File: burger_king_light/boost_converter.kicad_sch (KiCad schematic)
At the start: 14 parts, among them IC1 TPS55340PWPR

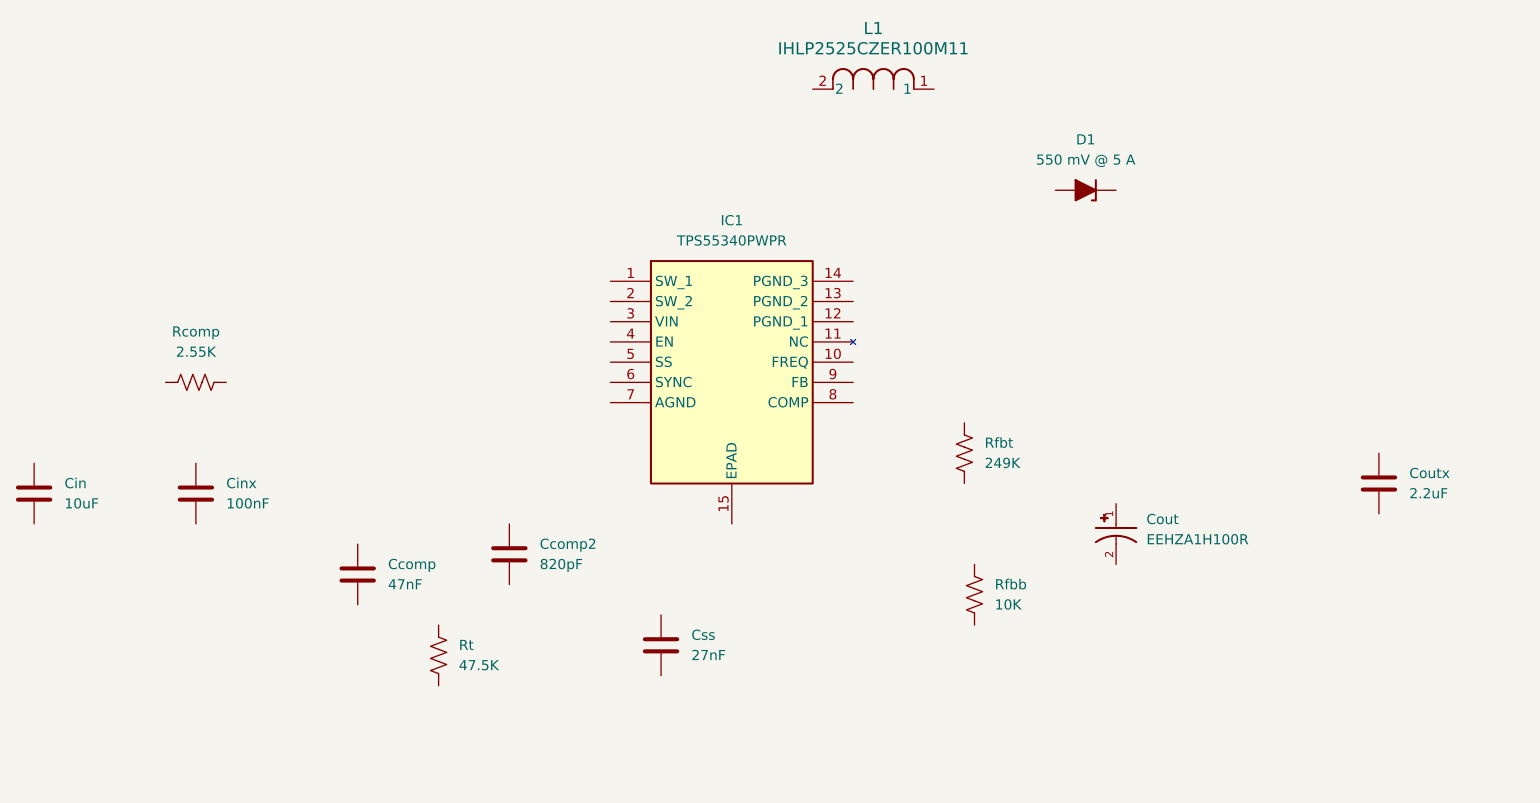
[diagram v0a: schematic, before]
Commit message: finished diagram
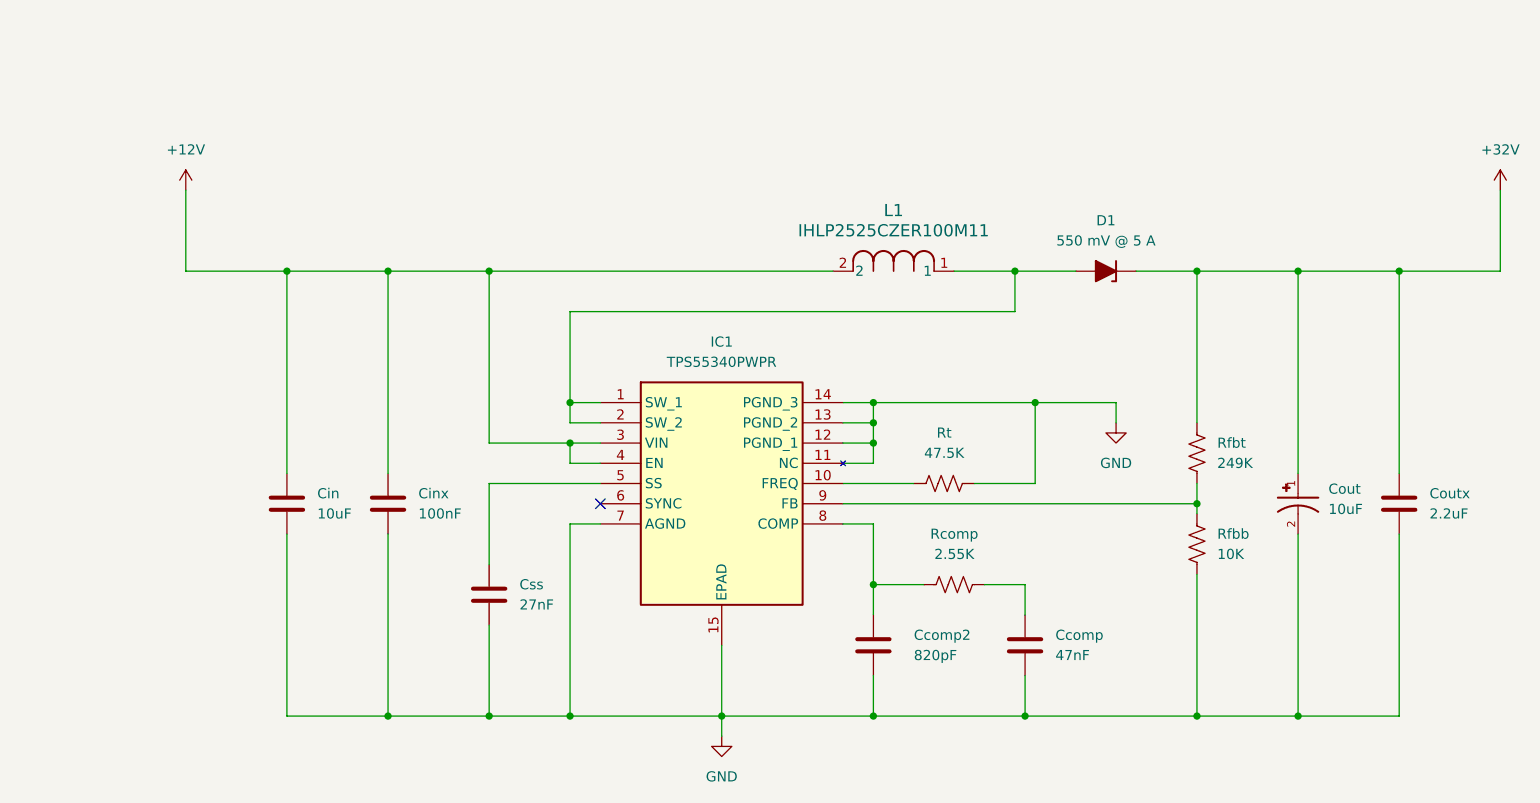
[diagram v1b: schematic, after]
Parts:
- Cout: value EEHZA1H100R -> 10uF
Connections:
- net +32V: now reaches Cout.1
- net +32V: now also Coutx.1, D1.1 (K), Rfbt.1
- net GND: now reaches Cout.2
- net GND: now also Ccomp.2, Ccomp2.2, Cin.2, Cinx.2, Coutx.2, Css.2, IC1.11 (NC), IC1.12 (PGND_1), IC1.13 (PGND_2), IC1.14 (PGND_3), IC1.15 (EPAD), IC1.7 (AGND), Rfbb.2, Rt.1
- net at Ccomp.1: now also Rcomp.2
- net at Rfbt.2: now also IC1.9 (FB), Rfbb.1
- net at Rcomp.1: now also Ccomp2.1, IC1.8 (COMP)
- net at L1.1: now also D1.2 (A), IC1.1 (SW_1), IC1.2 (SW_2)
- net +12V: now reaches L1.2
- net +12V: now also Cin.1, Cinx.1, IC1.3 (VIN), IC1.4 (EN)
- net at Rt.2: now also IC1.10 (FREQ)
- net at Css.1: now also IC1.5 (SS)
- no-connect marks 0 -> 1
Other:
- moved on the sheet: Ccomp, Ccomp2, Cin, Cinx, Cout, Coutx, Css, D1, IC1, L1, Rcomp, Rfbb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
